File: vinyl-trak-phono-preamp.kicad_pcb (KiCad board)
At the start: 2 copper layers, 64 x 31.5 mm, 67 parts, among them J2 Screw_Terminal_01x03, J3 Screw_Terminal_01x02, J4 Screw_Terminal_01x02, Q1 2N3906, Q10 2N3906, Q11 JFE2140D, Q12 2N5089, Q13 2N3904, Q14 2N3904, Q15 2N5089, Q16 2N5087, Q17 2N5087, Q18 2N5089, Q19 2N5089, Q2 2N3904, Q20 2N5087, Q21 2N5089, Q3 2N3906, Q4 2N3906, Q5 2N3904, Q6 2N3904, Q7 2N3904, Q8 2N3906, Q9 2N3904, U1 OPA2134

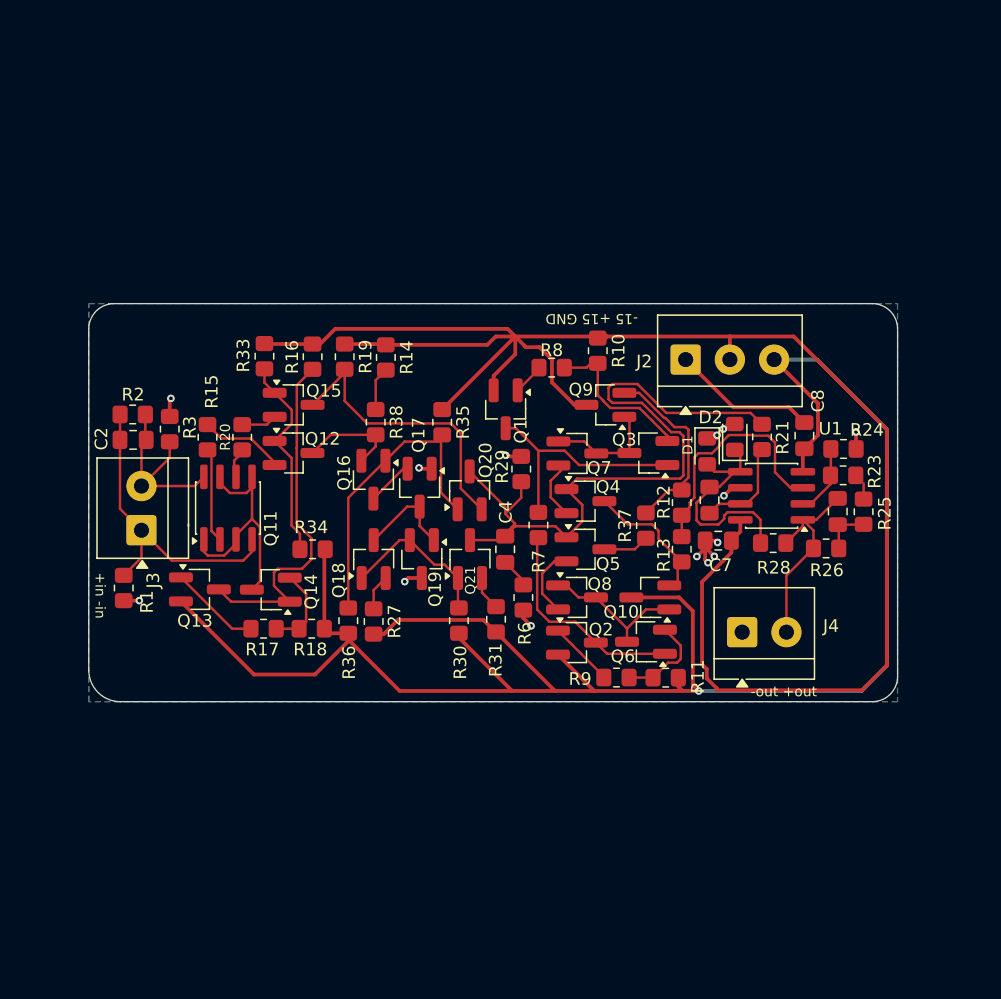
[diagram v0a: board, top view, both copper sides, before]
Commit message: Revision 0.1
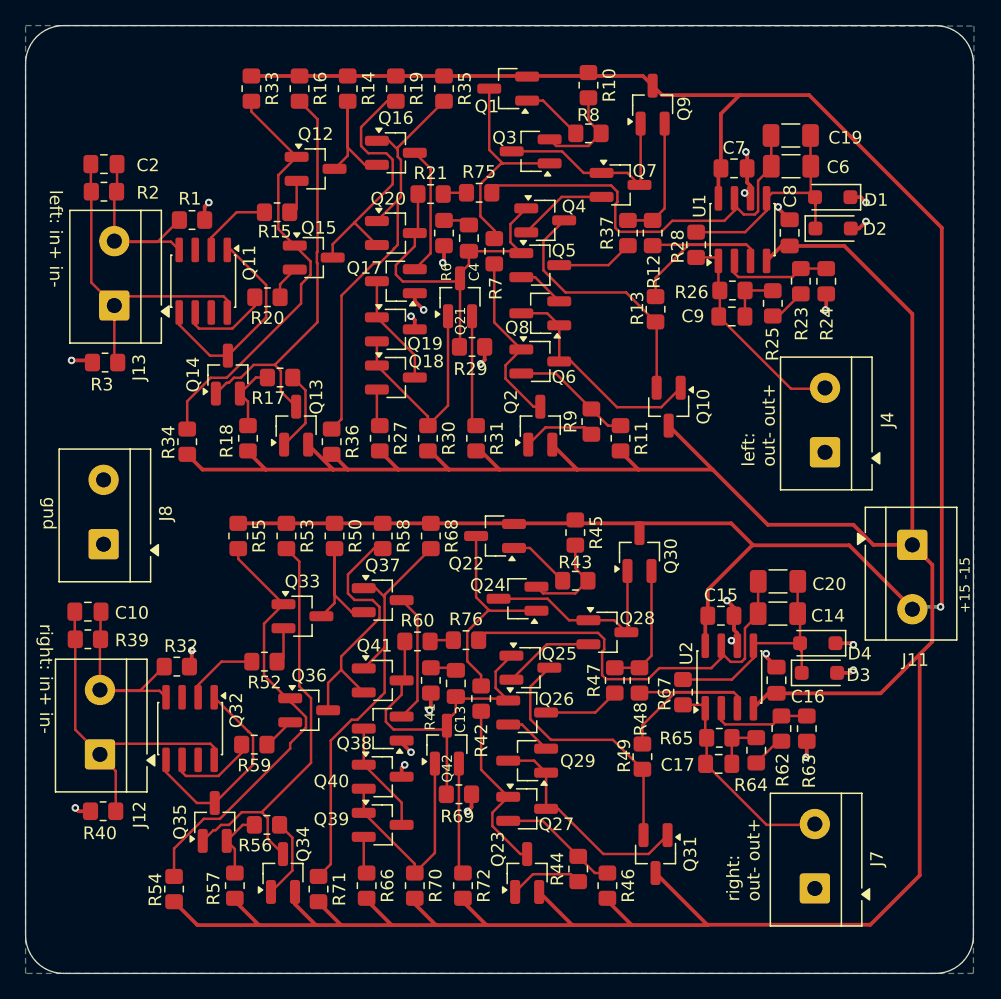
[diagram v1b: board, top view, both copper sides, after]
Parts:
- removed J2: Screw_Terminal_01x03, TerminalBlock_4Ucon:TerminalBlock_4Ucon_1x03_P3.50mm_Horizontal
- removed J3: Screw_Terminal_01x02, TerminalBlock_4Ucon:TerminalBlock_4Ucon_1x02_P3.50mm_Horizontal
- removed R38: 1, Resistor_SMD:R_0805_2012Metric_Pad1.20x1.40mm_HandSolder
- added C10: 100p, Capacitor_SMD:C_0805_2012Metric_Pad1.18x1.45mm_HandSolder, F.Cu at (74.9, 96.4)
- added C13: 0.015u, Capacitor_SMD:C_0805_2012Metric_Pad1.18x1.45mm_HandSolder, F.Cu at (104.0, 102.1)
- added C14: .47u, Capacitor_SMD:C_1206_3216Metric_Pad1.33x1.80mm_HandSolder, F.Cu at (129.5, 96.5)
- added C15: 10n, Capacitor_SMD:C_0805_2012Metric_Pad1.18x1.45mm_HandSolder, F.Cu at (125.0, 96.7)
- added C16: 10n, Capacitor_SMD:C_0805_2012Metric_Pad1.18x1.45mm_HandSolder, F.Cu at (129.4, 101.8)
- added C17: 0.020u, Capacitor_SMD:C_0805_2012Metric_Pad1.18x1.45mm_HandSolder, F.Cu at (124.8, 108.4)
- added C19: .47u, Capacitor_SMD:C_1206_3216Metric_Pad1.33x1.80mm_HandSolder, F.Cu at (130.5, 58.7)
- added C20: .47u, Capacitor_SMD:C_1206_3216Metric_Pad1.33x1.80mm_HandSolder, F.Cu at (129.5, 94.0)
- added D3: 1N4148W, Diode_SMD:D_SOD-123F, F.Cu at (132.7, 98.9)
- added D4: 1N4148W, Diode_SMD:D_SOD-123F, F.Cu at (132.8, 101.2)
- added J11: Screw_Terminal_01x02, Library:TerminalBlock_4Ucon_1x02_P5mm_Horizontal, F.Cu at (140.2, 91.6)
- added J12: Screw_Terminal_01x02, Library:TerminalBlock_4Ucon_1x02_P5mm_Horizontal, F.Cu at (75.9, 107.1)
- added J13: Screw_Terminal_01x02, Library:TerminalBlock_4Ucon_1x02_P5mm_Horizontal, F.Cu at (77.0, 71.6)
- added J7: Screw_Terminal_01x02, Library:TerminalBlock_4Ucon_1x02_P5mm_Horizontal, F.Cu at (132.5, 117.7)
- added J8: Screw_Terminal_01x02, Library:TerminalBlock_4Ucon_1x02_P5mm_Horizontal, F.Cu at (76.2, 90.5)
- added Q22: 2N3906, Library:SOT-23_Handsoldering-adjusted-pinout, F.Cu at (107.1, 90.4)
- added Q23: 2N3904, Library:SOT-23_Handsoldering-adjusted-pinout, F.Cu at (109.7, 117.1)
- added Q24: 2N3906, Library:SOT-23_Handsoldering-adjusted-pinout, F.Cu at (108.9, 95.4)
- added Q25: 2N3906, Library:SOT-23_Handsoldering-adjusted-pinout, F.Cu at (109.9, 100.8)
- added Q26: 2N3904, Library:SOT-23_Handsoldering-adjusted-pinout, F.Cu at (109.7, 104.4)
- added Q27: 2N3904, Library:SOT-23_Handsoldering-adjusted-pinout, F.Cu at (109.7, 112.0)
- added Q28: 2N3904, Library:SOT-23_Handsoldering-adjusted-pinout, F.Cu at (116.0, 98.0)
- added Q29: 2N3906, Library:SOT-23_Handsoldering-adjusted-pinout, F.Cu at (109.7, 108.2)
- added Q30: 2N3904, Library:SOT-23_Handsoldering-adjusted-pinout, F.Cu at (118.6, 91.7)
- added Q31: 2N3906, Library:SOT-23_Handsoldering-adjusted-pinout, F.Cu at (119.8, 115.6)
- added Q32: JFE2140D, Package_SO:SOIC-8_3.9x4.9mm_P1.27mm, F.Cu at (83.0, 105.6)
- added Q33: 2N5089, Library:SOT-23_Handsoldering-adjusted-pinout, F.Cu at (91.9, 96.7)
- added Q34: 2N3904, Library:SOT-23_Handsoldering-adjusted-pinout, F.Cu at (90.4, 117.1)
- added Q35: 2N3904, Library:SOT-23_Handsoldering-adjusted-pinout, F.Cu at (85.0, 113.0)
- added Q36: 2N5089, Library:SOT-23_Handsoldering-adjusted-pinout, F.Cu at (92.4, 104.2)
- added Q37: 2N5087, Library:SOT-23_Handsoldering-adjusted-pinout, F.Cu at (98.3, 95.5)
- added Q38: 2N5087, Library:SOT-23_Handsoldering-adjusted-pinout, F.Cu at (98.3, 105.6)
- added Q39: 2N5089, Library:SOT-23_Handsoldering-adjusted-pinout, F.Cu at (98.3, 113.2)
- added Q40: 2N5089, Library:SOT-23_Handsoldering-adjusted-pinout, F.Cu at (98.3, 109.4)
- added Q41: 2N5087, Library:SOT-23_Handsoldering-adjusted-pinout, F.Cu at (98.3, 101.8)
- added Q42: 2N5089, Library:SOT-23_Handsoldering-adjusted-pinout, F.Cu at (103.3, 106.9)
- added R32: 100k, Resistor_SMD:R_0805_2012Metric_Pad1.20x1.40mm_HandSolder, F.Cu at (82.0, 100.7)
- added R39: 18k, Resistor_SMD:R_0805_2012Metric_Pad1.20x1.40mm_HandSolder, F.Cu at (74.9, 98.6)
- added R40: 100k, Resistor_SMD:R_0805_2012Metric_Pad1.20x1.40mm_HandSolder, F.Cu at (76.1, 112.2)
- added R41: 1k37, Resistor_SMD:R_0805_2012Metric_Pad1.20x1.40mm_HandSolder, F.Cu at (102.1, 101.8)
- added R42: 205k, Resistor_SMD:R_0805_2012Metric_Pad1.20x1.40mm_HandSolder, F.Cu at (106.0, 103.3)
- added R43: 220, Resistor_SMD:R_0805_2012Metric_Pad1.20x1.40mm_HandSolder, F.Cu at (113.5, 93.9)
- added R44: 220, Resistor_SMD:R_0805_2012Metric_Pad1.20x1.40mm_HandSolder, F.Cu at (113.7, 116.7)
- added R45: 604, Resistor_SMD:R_0805_2012Metric_Pad1.20x1.40mm_HandSolder, F.Cu at (113.5, 90.1)
- added R46: 604, Resistor_SMD:R_0805_2012Metric_Pad1.20x1.40mm_HandSolder, F.Cu at (116.0, 118.1)
- added R47: 1, Resistor_SMD:R_0805_2012Metric_Pad1.20x1.40mm_HandSolder, F.Cu at (116.6, 101.8)
- added R48: 220, Resistor_SMD:R_0805_2012Metric_Pad1.20x1.40mm_HandSolder, F.Cu at (118.6, 101.8)
- added R49: 220, Resistor_SMD:R_0805_2012Metric_Pad1.20x1.40mm_HandSolder, F.Cu at (118.8, 107.8)
- added R50: 1k47, Resistor_SMD:R_0805_2012Metric_Pad1.20x1.40mm_HandSolder, F.Cu at (94.4, 90.4)
- added R52: 100, Resistor_SMD:R_0805_2012Metric_Pad1.20x1.40mm_HandSolder, F.Cu at (88.9, 100.3)
- added R53: 71k5, Resistor_SMD:R_0805_2012Metric_Pad1.20x1.40mm_HandSolder, F.Cu at (90.6, 90.4)
- added R54: 56k2, Resistor_SMD:R_0805_2012Metric_Pad1.20x1.40mm_HandSolder, F.Cu at (81.7, 118.3)
- added R55: 20.5k, Resistor_SMD:R_0805_2012Metric_Pad1.20x1.40mm_HandSolder, F.Cu at (86.8, 90.4)
- added R56: 220, Resistor_SMD:R_0805_2012Metric_Pad1.20x1.40mm_HandSolder, F.Cu at (89.1, 113.2)
- added R57: 160, Resistor_SMD:R_0805_2012Metric_Pad1.20x1.40mm_HandSolder, F.Cu at (86.6, 118.1)
- added R58: 1k47, Resistor_SMD:R_0805_2012Metric_Pad1.20x1.40mm_HandSolder, F.Cu at (98.3, 90.4)
- added R59: 100, Resistor_SMD:R_0805_2012Metric_Pad1.20x1.40mm_HandSolder, F.Cu at (88.1, 106.9)
- added R60: 56k2, Resistor_SMD:R_0805_2012Metric_Pad1.20x1.40mm_HandSolder, F.Cu at (101.0, 98.7)
- added R62: 1k47, Resistor_SMD:R_0805_2012Metric_Pad1.20x1.40mm_HandSolder, F.Cu at (129.8, 105.6)
- added R63: 1k47, Resistor_SMD:R_0805_2012Metric_Pad1.20x1.40mm_HandSolder, F.Cu at (131.8, 105.6)
- added R64: 15k0, Resistor_SMD:R_0805_2012Metric_Pad1.20x1.40mm_HandSolder, F.Cu at (127.8, 107.3)
- added R65: 162k, Resistor_SMD:R_0805_2012Metric_Pad1.20x1.40mm_HandSolder, F.Cu at (124.9, 106.4)
- added R66: 1k78, Resistor_SMD:R_0805_2012Metric_Pad1.20x1.40mm_HandSolder, F.Cu at (97.0, 118.1)
- added R67: 1Meg, Resistor_SMD:R_0805_2012Metric_Pad1.20x1.40mm_HandSolder, F.Cu at (122.0, 102.7)
- added R68: 33.2k, Resistor_SMD:R_0805_2012Metric_Pad1.20x1.40mm_HandSolder, F.Cu at (102.1, 90.4)
- added R69: 3k83, Resistor_SMD:R_0805_2012Metric_Pad1.20x1.40mm_HandSolder, F.Cu at (104.3, 110.8)
- added R70: 47.5k, Resistor_SMD:R_0805_2012Metric_Pad1.20x1.40mm_HandSolder, F.Cu at (100.8, 118.1)
- added R71: 115k, Resistor_SMD:R_0805_2012Metric_Pad1.20x1.40mm_HandSolder, F.Cu at (93.2, 118.3)
- added R72: 1k78, Resistor_SMD:R_0805_2012Metric_Pad1.20x1.40mm_HandSolder, F.Cu at (104.6, 118.1)
- added R75: 1, Resistor_SMD:R_0805_2012Metric_Pad1.20x1.40mm_HandSolder, F.Cu at (105.9, 63.2)
- added R76: 1, Resistor_SMD:R_0805_2012Metric_Pad1.20x1.40mm_HandSolder, F.Cu at (104.8, 98.6)
- added U2: OPA2134, Package_SO:SOIC-8_3.9x4.9mm_P1.27mm, F.Cu at (125.7, 101.5)
- C6: value 1u -> .47u; footprint Capacitor_SMD:C_0805_2012Metric_Pad1.18x1.45mm_HandSolder -> Capacitor_SMD:C_1206_3216Metric_Pad1.33x1.80mm_HandSolder
- D1, D2: value D -> 1N4148W; footprint Diode_SMD:D_0805_2012Metric_Pad1.15x1.40mm_HandSolder -> Diode_SMD:D_SOD-123F
- J4: footprint TerminalBlock_4Ucon:TerminalBlock_4Ucon_1x02_P3.50mm_Horizontal -> Library:TerminalBlock_4Ucon_1x02_P5mm_Horizontal
- R10, R11: value 600 -> 604
- R12, R13: value 215 -> 220
- R16: value 70k -> 71k5
- R23, R24: value 1470 -> 1k47
- R30: value 47k -> 47.5k
- R33: value 20k -> 20.5k
- R34: value 57k -> 56k2
- R35: value 33k -> 33.2k
- R7: value 200k -> 205k
- moved R21 32.5 mm to (102.0, 63.3), turned to 0 degrees
- moved R1 29.6 mm to (83.2, 65.4), turned to 180 degrees
- moved R6 29.5 mm to (103.1, 66.4)
- moved C7 29.5 mm to (126.1, 61.3), turned to 180 degrees
- moved C6 27.2 mm to (130.6, 61.1), turned to 180 degrees
- moved R35 26.4 mm to (103.1, 55.0)
- moved Q16 25.9 mm to (99.3, 60.1), turned to 0 degrees
- moved Q3 25.6 mm to (110.0, 60.0)
- moved Q1 25.4 mm to (108.2, 55.0), turned to 180 degrees
- moved C4 24.8 mm to (105.1, 66.8), turned to 90 degrees
- moved R28 24.4 mm to (123.1, 67.3), turned to -90 degrees
- moved Q9 24.0 mm to (119.6, 56.3), turned to 90 degrees
- moved Q6 23.7 mm to (110.7, 76.6), turned to 0 degrees
- moved R37 23.2 mm to (117.7, 66.4)
- moved Q5 22.8 mm to (110.7, 69.0)
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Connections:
- net /buffer renamed /phono-in-left/buffer
- net /buffer+ renamed /phono-in-left/buffer-
- net /cartridge+ renamed /l-in-
- net /cartridge- renamed /l-in+
- net /cascode renamed /phono-in-left/cascode
- net /out renamed /l-out
- C6 pad 2: Net-(C6-Pad2) -> Net-(C19-Pad2)
- Q11 pad 1: Net-(Q11C-VCH) -> Net-(Q14-C)
- Q11 pad 3: Net-(Q11C-VCH) -> unconnected-(Q11C-VCH-Pad3)
- Q11 pad 5: Net-(Q11C-VCH) -> Net-(Q14-C)
- Q11 pad 7: Net-(Q11C-VCH) -> unconnected-(Q11C-VCL-Pad7)
- Q12 pad 1: /buffer- -> /phono-in-left/buffer+
- Q14 pad 1: Net-(Q11C-VCH) -> Net-(Q14-C)
- Q16 pad 3: /buffer- -> /phono-in-left/buffer+
- R14 pad 2: Net-(R14-Pad2) -> /phono-in-left/buffer+
- R21 pad 2: Net-(C6-Pad2) -> Net-(R21-Pad2)
- U1 pad 7: Net-(C6-Pad2) -> Net-(C19-Pad2)
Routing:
- net -15: track 152.0 -> 247.5 mm, vias 1 -> 0
- net Net-(Q33-B): track 0.00 -> 34.7 mm
- net Net-(Q37-B): track 0.00 -> 34.2 mm
- net Net-(C19-Pad2): track 0.00 -> 33.1 mm
- net Net-(C14-Pad2): track 0.00 -> 33.1 mm
- net Net-(Q34-C): track 0.00 -> 32.9 mm
- net /phono-in-left/cascode: track 57.1 -> 27.6 mm
- net /phono-in-right/cascode: track 0.00 -> 27.7 mm
- net +15V: track 138.6 -> 165.8 mm, vias 0 -> 1
- net /r-in-: track 0.00 -> 26.3 mm
- net /phono-in-right/buffer-: track 0.00 -> 20.4 mm
- net Net-(Q25-C): track 0.00 -> 20.3 mm
- net Net-(Q11C-VCH): track 19.3 -> 0.00 mm
- net /phono-in-right/buffer: track 0.00 -> 18.6 mm
- net Net-(Q27-C): track 0.00 -> 18.0 mm
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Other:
- board size 64 x 31.5 mm -> 75 x 75 mm
- board text added: "+15 -15"
- board text added: "VinylTrak MM Phono Preamp Input Stage - Rev. 0.1 Designed by Bob Cordell Created by Brian Lubeski • 2026-05"
- board text added: "gnd"
- board text added: "left: in+ in-"
- board text added: "left: out- out+"
- board text added: "right: in+ in-"
- board text added: "right: out- out+"
- board text removed: "+in -in"
- board text removed: "-15 +15 GND"
- board text removed: "-out +out"
